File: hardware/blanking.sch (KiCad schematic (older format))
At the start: 21 parts, among them U5 74HC4538, U6 74HC4538, U7 LM1881, U8 CD4053B

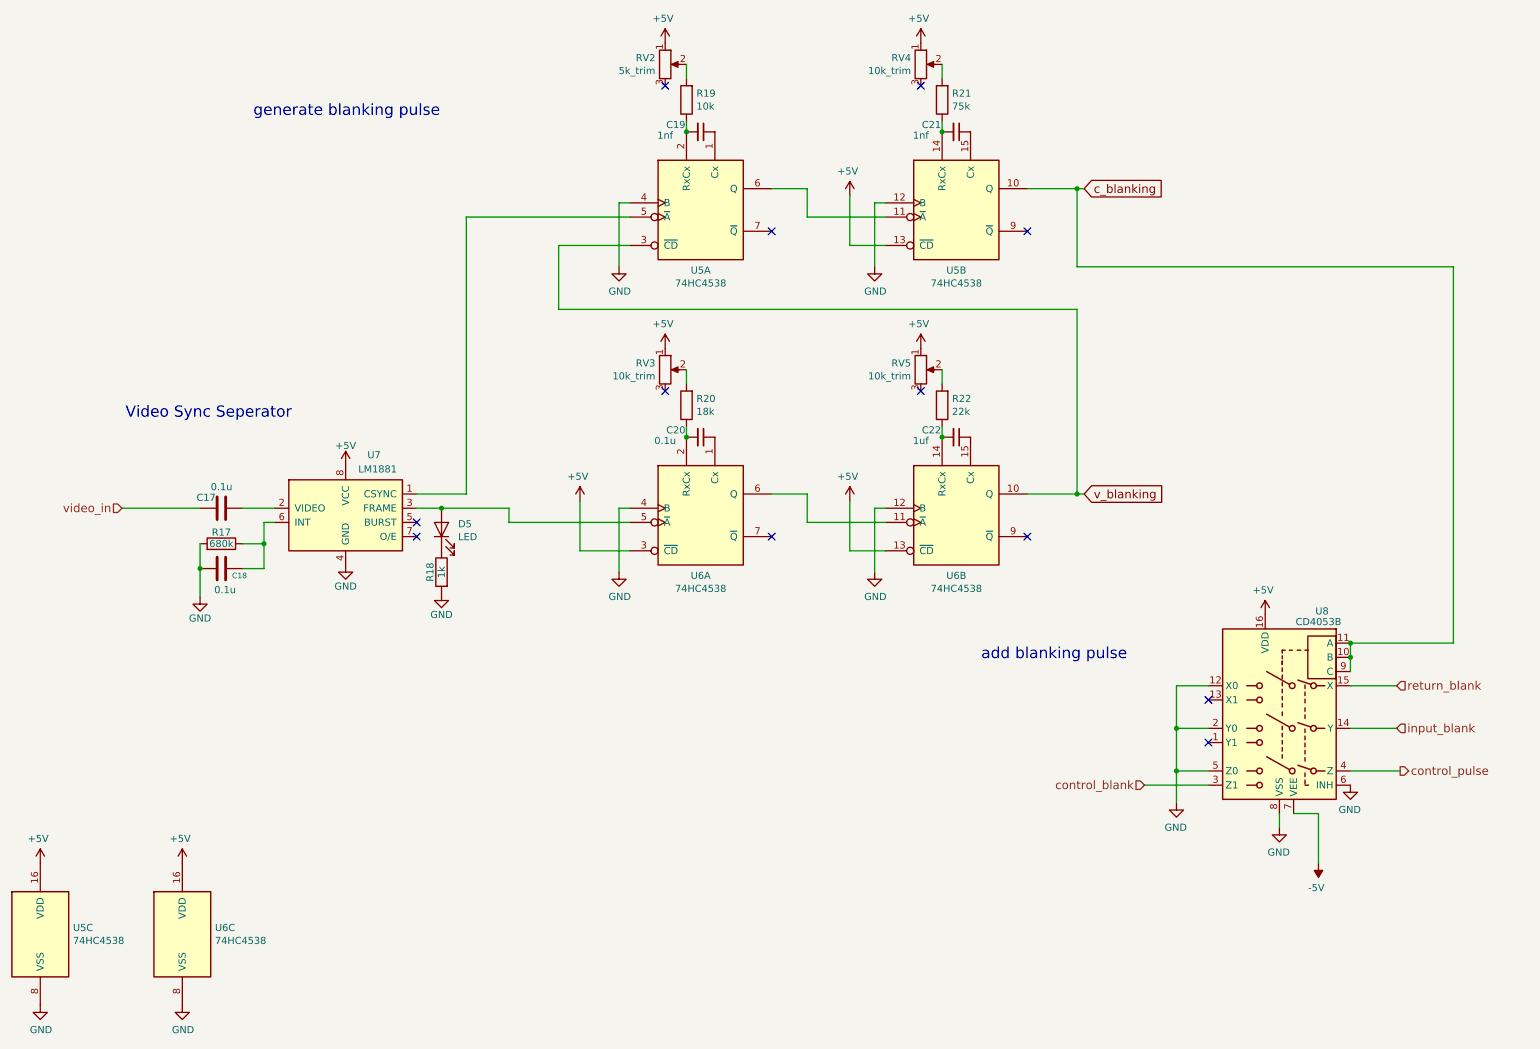
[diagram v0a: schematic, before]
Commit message: made final? fixes to the board
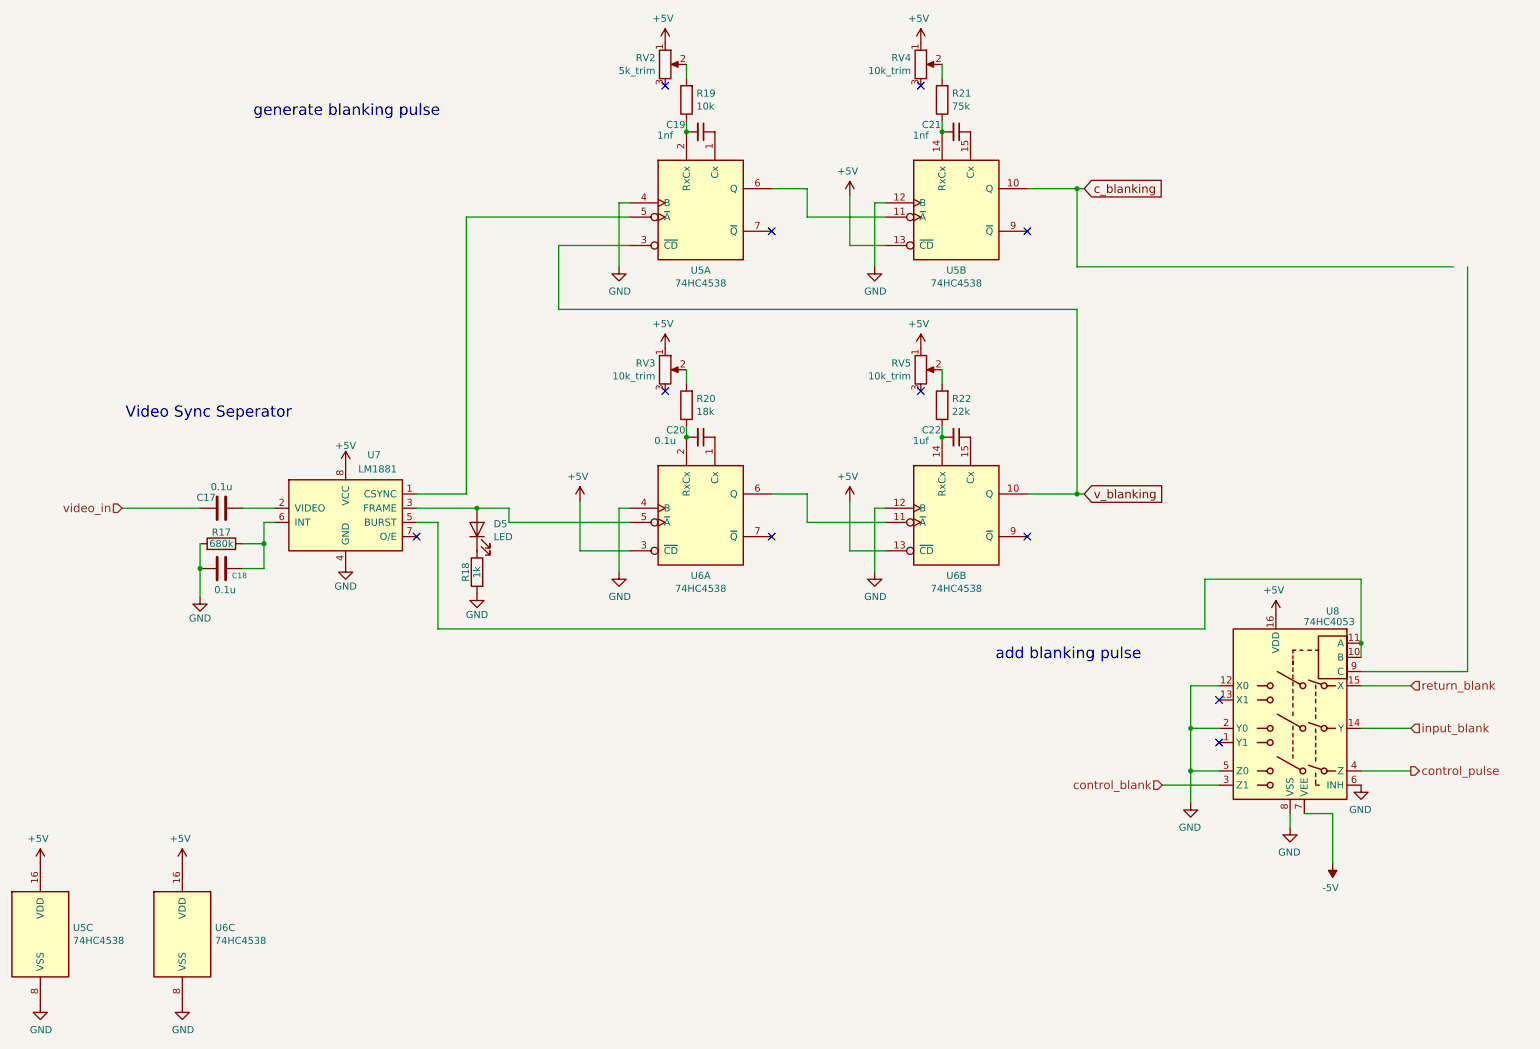
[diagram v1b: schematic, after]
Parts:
- U8: value CD4053B -> 74HC4053
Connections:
- net c_blanking: no longer U8.10 (B), U8.11 (A), U8.9 (C)
- net at U7.5 (BURST): now also U8.10 (B), U8.11 (A)
- no-connect marks 12 -> 11
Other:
- moved on the sheet: D5, R18, U8
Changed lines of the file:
@@
 L Sync-Ope-proto-rescue:R-Sync-Ope-proto-Sync-Ope-proto-rescue R?
 U 1 1 5FDF1AC6
-P 3675 4450
+P 3925 4450
 AR Path="/5FDF1AC6" Ref="R?"  Part="1"
 AR Path="/5FDD6789/5FDF1AC6" Ref="R18"  Part="1"
-F 0 "R18" V 3755 4450 50  0000 C CNN
-F 1 "1k" V 3675 4450 50  0000 C CNN
-F 2 "Resistor_THT:R_Axial_DIN0204_L3.6mm_D1.6mm_P7.62mm_Horizontal" V 3605 4450 50  0001 C CNN
-F 3 "" H 3675 4450 50  0001 C CNN
-	1    3675 4450
+F 0 "R18" V 4005 4450 50  0000 C CNN
+F 1 "1k" V 3925 4450 50  0000 C CNN
+F 2 "Resistor_THT:R_Axial_DIN0204_L3.6mm_D1.6mm_P7.62mm_Horizontal" V 3855 4450 50  0001 C CNN
+F 3 "" H 3925 4450 50  0001 C CNN
+	1    3925 4450
 	-1   0    0    -1
 $EndComp
@@
 L Sync-Ope-proto-rescue:LED-Device D?
 U 1 1 5FDF1ACC
-P 3675 4150
+P 3925 4150
 AR Path="/5FDF1ACC" Ref="D?"  Part="1"
 AR Path="/5FDD6789/5FDF1ACC" Ref="D5"  Part="1"
-F 0 "D5" V 3714 4033 50  0000 R CNN
-F 1 "LED" V 3623 4033 50  0000 R CNN
-F 2 "LED_THT:LED_D3.0mm" H 3675 4150 50  0001 C CNN
-F 3 "~" H 3675 4150 50  0001 C CNN
-	1    3675 4150
+F 0 "D5" V 3964 4033 50  0000 R CNN
+F 1 "LED" V 3873 4033 50  0000 R CNN
+F 2 "LED_THT:LED_D3.0mm" H 3925 4150 50  0001 C CNN
+F 3 "~" H 3925 4150 50  0001 C CNN
+	1    3925 4150
 	0    -1   -1   0
 $EndComp
 Text HLabel 1425 4000 0    60   Input ~ 0
 video_in
-Text HLabel 10400 5550 2    60   Input ~ 0
+Text HLabel 10500 5550 2    60   Input ~ 0
 input_blank
-Text HLabel 10400 5250 2    60   Input ~ 0
+Text HLabel 10500 5250 2    60   Input ~ 0
 return_blank
-Text HLabel 10425 5850 2    60   Output ~ 0
+Text HLabel 10500 5850 2    60   Output ~ 0
 control_pulse
-Text HLabel 8625 5950 0    60   Input ~ 0
+Text HLabel 8750 5950 0    60   Input ~ 0
 control_blank
 $Comp
 L power:GND #PWR064
 U 1 1 5FDDBCAE
-P 9575 6250
-F 0 "#PWR064" H 9575 6000 50  0001 C CNN
-F 1 "GND" H 9580 6077 50  0000 C CNN
-F 2 "" H 9575 6250 50  0001 C CNN
-F 3 "" H 9575 6250 50  0001 C CNN
-	1    9575 6250
-	-1   0    0    -1
-$EndComp
-Wire Wire Line
-	9575 6250 9575 6150
+P 9650 6250
+F 0 "#PWR064" H 9650 6000 50  0001 C CNN
+F 1 "GND" H 9655 6077 50  0000 C CNN
+F 2 "" H 9650 6250 50  0001 C CNN
+F 3 "" H 9650 6250 50  0001 C CNN
+	1    9650 6250
+	-1   0    0    -1
+$EndComp
 $Comp
 L power:GND #PWR066
 U 1 1 5FDDBCB8
-P 10075 5950
-F 0 "#PWR066" H 10075 5700 50  0001 C CNN
-F 1 "GND" H 10080 5777 50  0000 C CNN
-F 2 "" H 10075 5950 50  0001 C CNN
-F 3 "" H 10075 5950 50  0001 C CNN
-	1    10075 5950
+P 10150 5950
+F 0 "#PWR066" H 10150 5700 50  0001 C CNN
+F 1 "GND" H 10155 5777 50  0000 C CNN
+F 2 "" H 10150 5950 50  0001 C CNN
+F 3 "" H 10150 5950 50  0001 C CNN
+	1    10150 5950
 	-1   0    0    -1
 $EndComp
@@
 L power:+5V #PWR063
 U 1 1 5FDDBCBE
-P 9475 4750
-F 0 "#PWR063" H 9475 4600 50  0001 C CNN
-F 1 "+5V" H 9490 4923 50  0000 C CNN
-F 2 "" H 9475 4750 50  0001 C CNN
-F 3 "" H 9475 4750 50  0001 C CNN
-	1    9475 4750
-	-1   0    0    -1
-$EndComp
-Connection ~ 10075 5050
-Connection ~ 10075 4950
-Wire Wire Line
-	10075 5050 10075 5150
-Wire Wire Line
-	10075 4950 10075 5050
-$Comp
-L Sync-Ope-proto-rescue:CD4053B-Analog_Switch U?
-U 1 1 5FDDBCD5
-P 9575 5450
-AR Path="/5FDDBCD5" Ref="U?"  Part="1"
-AR Path="/5FDD6789/5FDDBCD5" Ref="U8"  Part="1"
-F 0 "U8" H 9275 6175 50  0000 C CNN
-F 1 "CD4053B" H 9300 6100 50  0000 C CNN
-F 2 "Package_DIP:DIP-16_W7.62mm_LongPads" H 9725 4700 50  0001 L CNN
-F 3 "http://www.ti.com/lit/ds/symlink/cd4052b.pdf" H 9555 5650 50  0001 C CNN
-	1    9575 5450
-	-1   0    0    -1
-$EndComp
-Wire Wire Line
-	8850 5250 9075 5250
+P 9550 4750
+F 0 "#PWR063" H 9550 4600 50  0001 C CNN
+F 1 "+5V" H 9565 4923 50  0000 C CNN
+F 2 "" H 9550 4750 50  0001 C CNN
+F 3 "" H 9550 4750 50  0001 C CNN
+	1    9550 4750
+	-1   0    0    -1
+$EndComp
 $Comp
 L 74hc4538:74HC4538 U6
@@
 Wire Wire Line
 	6000 3900 6250 3900
-Wire Wire Line
-	10075 4950 10800 4950
 $Comp
 L 74hc4538:74HC4538 U5
@@
 $EndComp
 Connection ~ 5400 3500
-Wire Wire Line
-	10400 5250 10075 5250
-Wire Wire Line
-	10400 5550 10075 5550
-Wire Wire Line
-	9075 5550 8850 5550
-Wire Wire Line
-	8850 5550 8850 5250
 $Comp
 L power:GND #PWR062
 U 1 1 603048A2
-P 8850 6075
-F 0 "#PWR062" H 8850 5825 50  0001 C CNN
-F 1 "GND" H 8855 5902 50  0000 C CNN
-F 2 "" H 8850 6075 50  0001 C CNN
-F 3 "" H 8850 6075 50  0001 C CNN
-	1    8850 6075
-	-1   0    0    -1
-$EndComp
-Connection ~ 8850 5550
-NoConn ~ 9075 5350
-NoConn ~ 9075 5650
-Wire Wire Line
-	10425 5850 10075 5850
-Wire Wire Line
-	9075 5850 8850 5850
-Wire Wire Line
-	8850 5550 8850 5850
-Connection ~ 8850 5850
-Wire Wire Line
-	8850 5850 8850 6075
-Wire Wire Line
-	9075 5950 8625 5950
+P 8950 6075
+F 0 "#PWR062" H 8950 5825 50  0001 C CNN
+F 1 "GND" H 8955 5902 50  0000 C CNN
+F 2 "" H 8950 6075 50  0001 C CNN
+F 3 "" H 8950 6075 50  0001 C CNN
+	1    8950 6075
+	-1   0    0    -1
+$EndComp
 Wire Wire Line
 	1425 4000 1975 4000
@@
 	1    0    0    -1
 $EndComp
-NoConn ~ 3500 4100
 NoConn ~ 3500 4200
 $Comp
 L Sync-Ope-proto-rescue:GND-Sync-Ope-proto-Sync-Ope-proto-rescue #PWR?
 U 1 1 603992F4
-P 3675 4600
+P 3925 4600
 AR Path="/603992F4" Ref="#PWR?"  Part="1"
 AR Path="/5FDD6789/603992F4" Ref="#PWR050"  Part="1"
-F 0 "#PWR050" H 3675 4350 50  0001 C CNN
-F 1 "GND" H 3675 4450 50  0000 C CNN
-F 2 "" H 3675 4600 50  0001 C CNN
-F 3 "" H 3675 4600 50  0001 C CNN
-	1    3675 4600
+F 0 "#PWR050" H 3925 4350 50  0001 C CNN
+F 1 "GND" H 3925 4450 50  0000 C CNN
+F 2 "" H 3925 4600 50  0001 C CNN
+F 3 "" H 3925 4600 50  0001 C CNN
+	1    3925 4600
 	1    0    0    -1
 $EndComp
@@
 Text Notes 2350 1250 0    79   ~ 0
 generate blanking pulse
-Text Notes 7475 5075 0    79   ~ 0
+Text Notes 7575 5075 0    79   ~ 0
 add blanking pulse
 $Comp
 L power:-5V #PWR065
 U 1 1 60E7AA52
-P 9850 6500
-F 0 "#PWR065" H 9850 6600 50  0001 C CNN
-F 1 "-5V" H 9865 6673 50  0000 C CNN
-F 2 "" H 9850 6500 50  0001 C CNN
-F 3 "" H 9850 6500 50  0001 C CNN
-	1    9850 6500
+P 9950 6500
+F 0 "#PWR065" H 9950 6600 50  0001 C CNN
+F 1 "-5V" H 9965 6673 50  0000 C CNN
+F 2 "" H 9950 6500 50  0001 C CNN
+F 3 "" H 9950 6500 50  0001 C CNN
+	1    9950 6500
 	-1   0    0    1
 $EndComp
 Wire Wire Line
-	9850 6500 9850 6150
-Wire Wire Line
-	9850 6150 9675 6150
+	9950 6500 9950 6150
 $Comp
 L 74hc4538:74HC4538 U6
@@
 	7800 1750 8150 1750
 Wire Wire Line
-	3500 4000 3675 4000
-Connection ~ 3675 4000
-Wire Wire Line
-	3675 4000 4150 4000
-Wire Wire Line
 	3850 1950 5000 1950
 Wire Wire Line
@@
 	8150 2300 10800 2300
 Wire Wire Line
-	10800 2300 10800 4950
-Wire Wire Line
 	8200 1750 8150 1750
 Connection ~ 8150 1750
+Wire Wire Line
+	10900 2300 10900 5150
+Wire Wire Line
+	8950 5250 8950 5550
+Wire Wire Line
+	9150 5950 8750 5950
+Wire Wire Line
+	9150 5850 8950 5850
+Connection ~ 8950 5850
+Wire Wire Line
+	8950 5850 8950 6075
+NoConn ~ 9150 5650
+Wire Wire Line
+	9150 5550 8950 5550
+Connection ~ 8950 5550
+Wire Wire Line
+	8950 5550 8950 5850
+Wire Wire Line
+	8950 5250 9150 5250
+NoConn ~ 9150 5350
+Wire Wire Line
+	9650 6250 9650 6150
+Wire Wire Line
+	9750 6150 9950 6150
+Wire Wire Line
+	10150 5850 10500 5850
+Wire Wire Line
+	10500 5550 10150 5550
+Wire Wire Line
+	10500 5250 10150 5250
+$Comp
+L Sync-Ope-proto-rescue:CD4053B-Analog_Switch U?
+U 1 1 5FDDBCD5
+P 9650 5450
+AR Path="/5FDDBCD5" Ref="U?"  Part="1"
+AR Path="/5FDD6789/5FDDBCD5" Ref="U8"  Part="1"
+F 0 "U8" H 9350 6175 50  0000 C CNN
+F 1 "74HC4053" H 9375 6100 50  0000 C CNN
+F 2 "Package_DIP:DIP-16_W7.62mm_LongPads" H 9800 4700 50  0001 L CNN
+F 3 "http://www.ti.com/lit/ds/symlink/cd4052b.pdf" H 9630 5650 50  0001 C CNN
+	1    9650 5450
+	-1   0    0    -1
+$EndComp
+Wire Wire Line
+	10150 5150 10900 5150
+Connection ~ 3925 4000
+Wire Wire Line
+	3925 4000 4150 4000
+Wire Wire Line
+	3500 4000 3925 4000
+Wire Wire Line
+	3500 4100 3650 4100
+Wire Wire Line
+	3650 4100 3650 4850
+Wire Wire Line
+	3650 4850 9050 4850
+Wire Wire Line
+	9050 4850 9050 4500
+Wire Wire Line
+	9050 4500 10150 4500
+Wire Wire Line
+	10150 4500 10150 4950
+Wire Wire Line
+	10150 4950 10150 5050
+Connection ~ 10150 4950
 $EndSCHEMATC
